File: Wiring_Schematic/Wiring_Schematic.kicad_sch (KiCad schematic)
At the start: 11 parts, among them SW1 Jab_Button, SW2 Crouch_Button, SW3 Dash_Button, SW4 Jump_Button

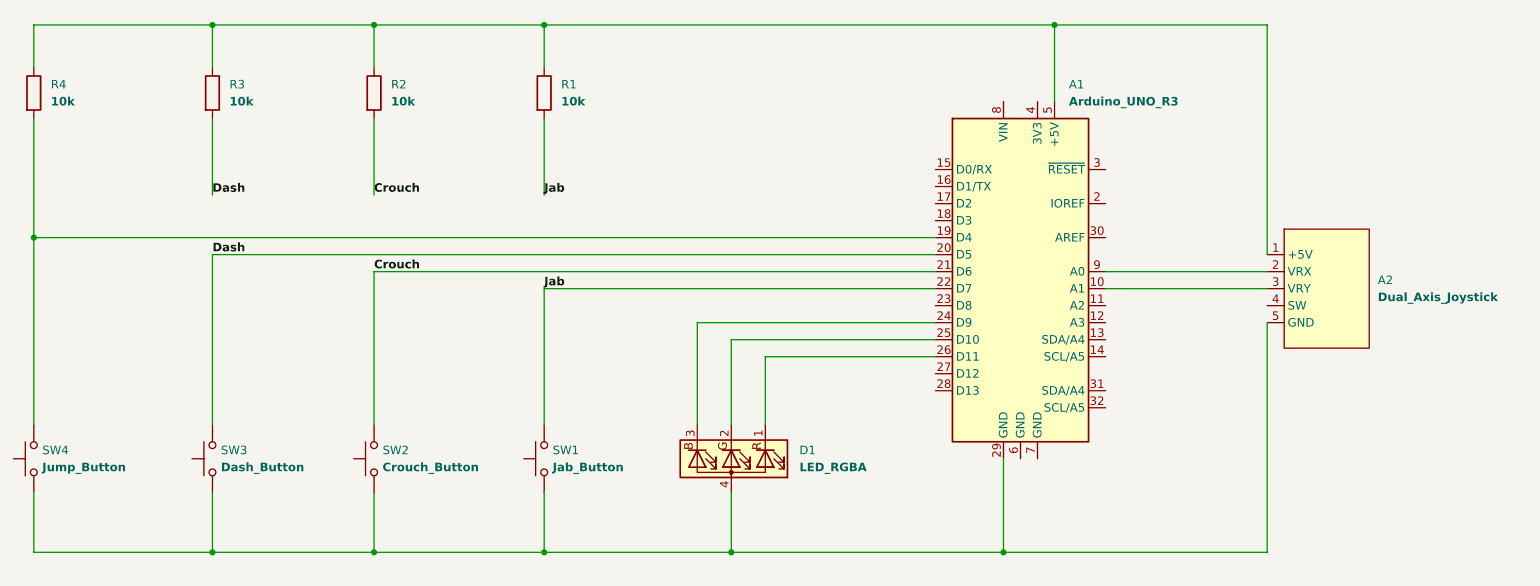
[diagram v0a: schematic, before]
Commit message: Squashed commit of the following:
commit 33099763b0ee2d5a55e8a517743b06c98f7c2c78
Merge: 906da59 90e3300
Author: Qfox1 <qn318632@dal.ca>
Date:   Wed Apr 1 09:51:05 2026 -0300

    Merge pull request #23 from MECH3905/Updating-KiCad

    Update Wiring_Schematic.kicad_sch

commit 90e33006c09e33d148ea8b2afd2a0e98a436d263
Author: Qfox1 <qn318632@dal.ca>
Date:   Wed Apr 1 09:50:24 2026 -0300

    Update Wiring_Schematic.kicad_sch

commit 906da5998a5aad2f887fd0f551d51e961ebdda60
Merge: c7f70ca 7aa0266
Author: Qfox1 <qn318632@dal.ca>
Date:   Tue Mar 31 13:27:45 2026 -0300

    Merge pull request #22 from MECH3905/Dash-images

    Added dash images

commit 7aa02663095d3a52a4dfee5a0e7541544721c1fb
Author: Qfox1 <qn318632@dal.ca>
Date:   Tue Mar 31 13:27:25 2026 -0300

    Added dash images

commit c7f70cac2cfec1cbe2acc37a1d87e9237dd0db6b
Author: Qfox1 <qn318632@dal.ca>
Date:   Tue Mar 31 13:17:21 2026 -0300

    Changed file names

commit b53879fd872a280acebafd178b68cac863f3b718
Merge: b0a6c40 df6cdc7
Author: Qfox1 <qn318632@dal.ca>
Date:   Tue Mar 31 13:15:17 2026 -0300

    Merge pull request #21 from MECH3905/End-screen

    End screen

commit df6cdc7418edd5f8c55060ab42896a0c1d49e2e2
Author: Qfox1 <qn318632@dal.ca>
Date:   Tue Mar 31 13:14:53 2026 -0300

    End game screens

commit 214c9ad2750c0d42b83944c13d8218d65170cfc4
Author: Qfox1 <qn318632@dal.ca>
Date:   Tue Mar 31 11:24:01 2026 -0300

    Squashed commit of the following:

    commit b0a6c40c548a6f97752e975c2658d9ccfaca288e
    Merge: 2728ccd dda4ca4
    Author: Qfox1 <qn318632@dal.ca>
    Date:   Tue Mar 31 11:17:12 2026 -0300

        Merge pull request #20 from MECH3905/Roasted-images

        Added roasted images

    commit dda4ca46d1f6f87b57c7988103e9a3d2f51da8c9
    Author: Qfox1 <qn318632@dal.ca>
    Date:   Tue Mar 31 11:16:48 2026 -0300

        Added roasted images

    commit 2728ccd58e093a41ce34cda207a2be2a120341fb
    Merge: f57d57b 3b8008a
    Author: Qfox1 <qn318632@dal.ca>
    Date:   Mon Mar 30 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
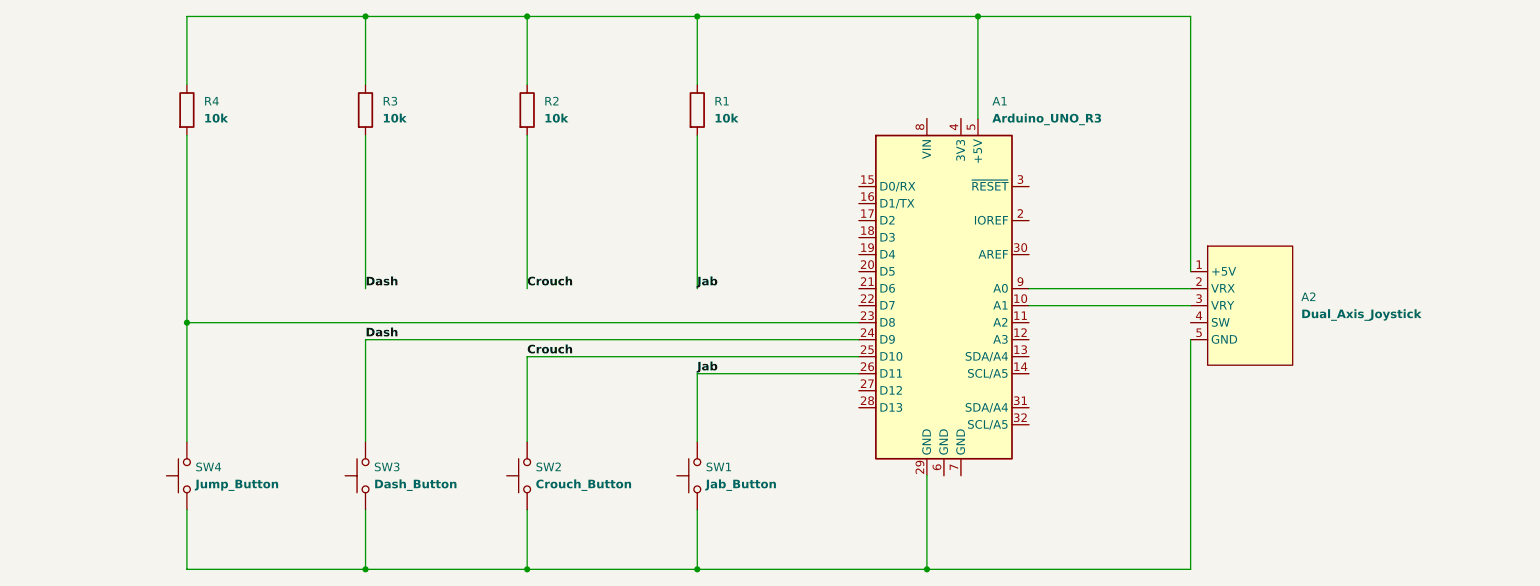
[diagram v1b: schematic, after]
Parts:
- removed D1: LED_RGBA, symbol Device:LED_RGBA
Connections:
- net Crouch: now also A1.25 (D10); no longer A1.21 (D6)
- net Dash: now also A1.24 (D9); no longer A1.20 (D5)
- net Jab: now also A1.26 (D11); no longer A1.22 (D7)
- net at R4.2, SW4.2: now also A1.23 (D8); no longer A1.19 (D4)
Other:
- title: MECH3905 Milestone 1 Controller Wiring Schematic -> MECH3905 Term Project Controller Wiring Schematic
- moved on the sheet: A1, A2, R1, R2, R3, R4, SW1, SW2, SW3, SW4
